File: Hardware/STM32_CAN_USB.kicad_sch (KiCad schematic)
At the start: 28 parts, among them J1 USB_C_Receptacle_USB2.0_14P, J2 SWD, J3 CAN Connector, J4 JP1, SW1 RESET, U1 AP2112K-3.3, U2 STM32F103C8Tx, U3 SN65HVD230, Y1 8Mhz

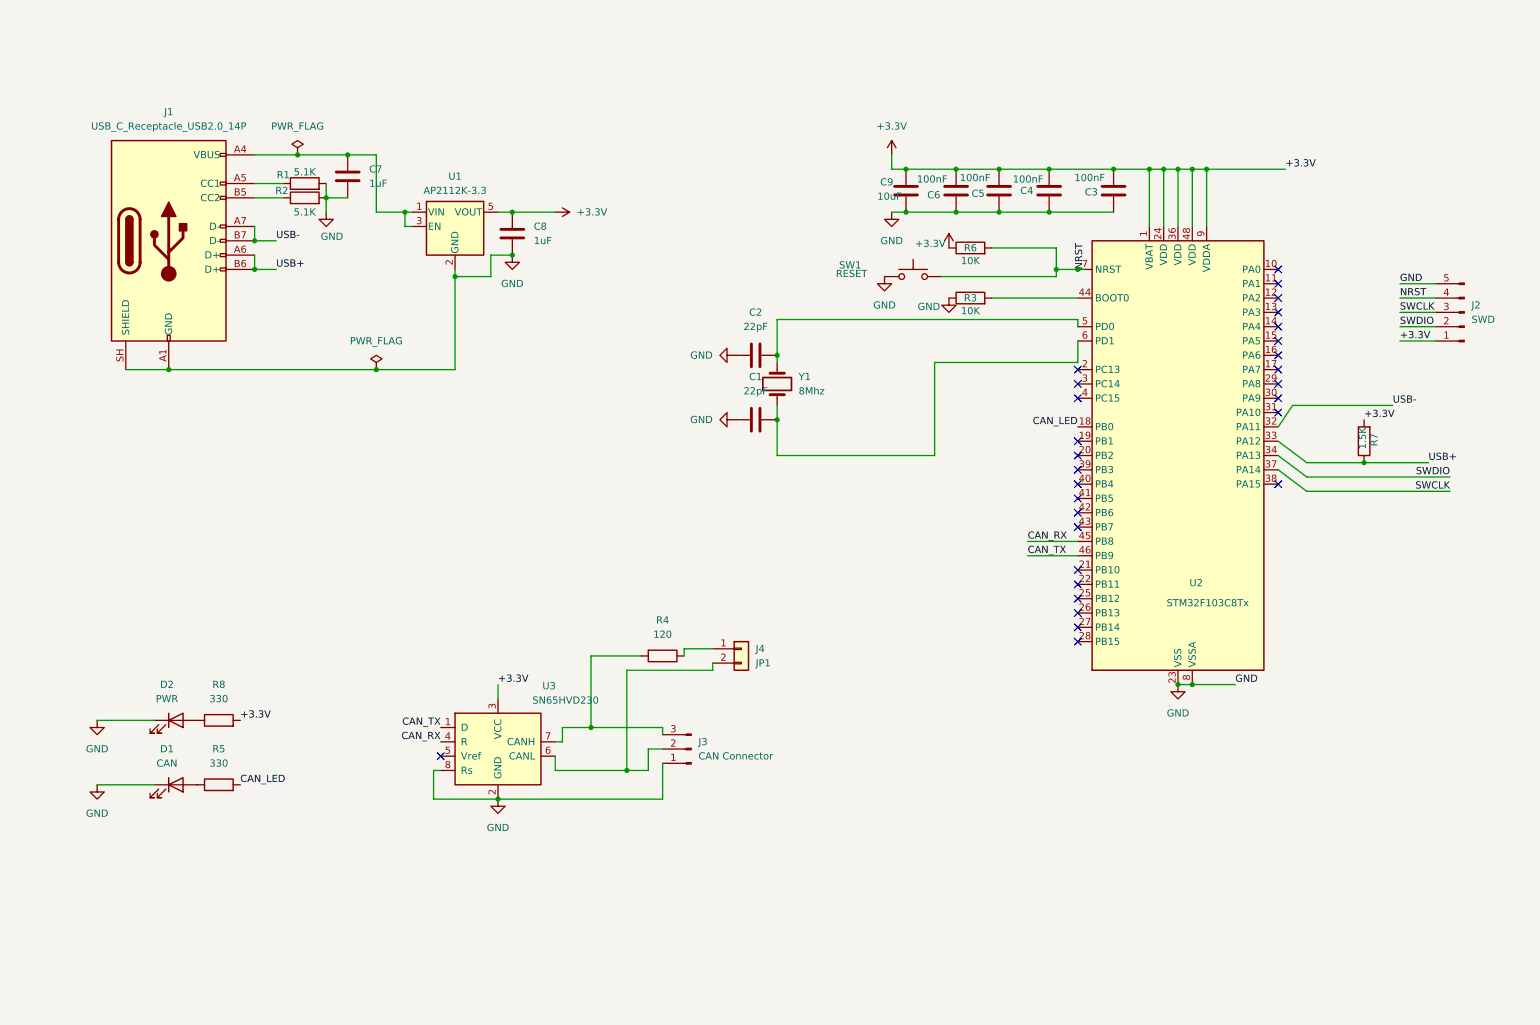
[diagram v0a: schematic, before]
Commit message: Replace project with updated design
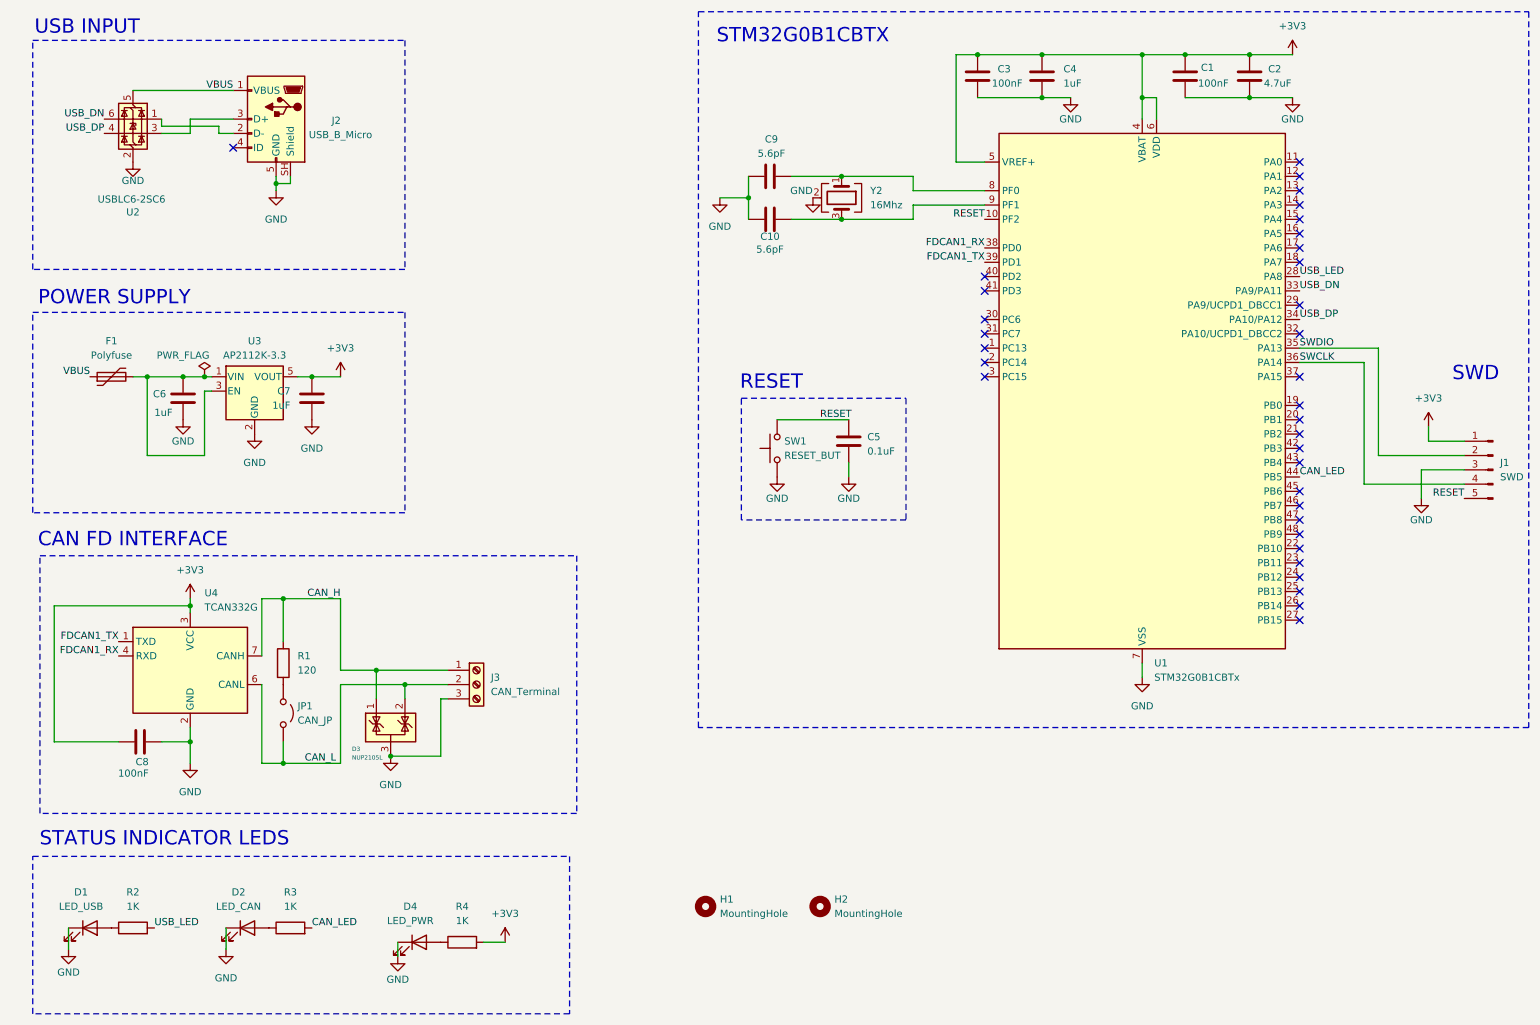
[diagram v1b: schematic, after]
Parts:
- removed J1: USB_C_Receptacle_USB2.0_14P, Connector_USB:USB_C_Receptacle_HRO_TYPE-C-31-M-12, symbol Connector:USB_C_Receptacle_USB2.0_14P
- removed J2: SWD, Connector_PinHeader_2.54mm:PinHeader_1x05_P2.54mm_Vertical, symbol Connector:Conn_01x05_Pin
- removed J3: CAN Connector, TerminalBlock_Phoenix:TerminalBlock_Phoenix_MKDS-1,5-3_1x03_P5.00mm_Horizontal, symbol Connector:Conn_01x03_Pin
- removed J4: JP1, Connector_PinHeader_2.54mm:PinHeader_1x02_P2.54mm_Vertical, symbol Connector_Generic:Conn_01x02
- removed R5, R8: 330, Resistor_SMD:R_0805_2012Metric, symbol Device:R
- removed R6: 10K, Resistor_SMD:R_0805_2012Metric, symbol Device:R
- removed R7: 1.5K, Resistor_SMD:R_0805_2012Metric, symbol Device:R
- removed U1: AP2112K-3.3, Package_TO_SOT_SMD:SOT-23-5, symbol Regulator_Linear:AP2112K-3.3
- removed U2: STM32F103C8Tx, Package_QFP:LQFP-48_7x7mm_P0.5mm, symbol MCU_ST_STM32F1:STM32F103C8Tx
- removed U3: SN65HVD230, Package_SO:SOIC-8_3.9x4.9mm_P1.27mm, symbol Interface_CAN_LIN:SN65HVD230
- removed Y1: 8Mhz, Crystal:Crystal_SMD_3225-4Pin_3.2x2.5mm, symbol Device:Crystal
- added C10: 5.6pF, Capacitor_SMD:C_0603_1608Metric, symbol Device:C
- added D3: NUP2105L, Package_TO_SOT_SMD:SOT-23, symbol Power_Protection:NUP2105L
- added D4: LED_PWR, LED_SMD:LED_0603_1608Metric, symbol Device:LED
- added F1: Polyfuse, Fuse:Fuse_1206_3216Metric, symbol Device:Polyfuse
- added H1, H2: MountingHole, MountingHole:MountingHole_2mm, symbol Mechanical:MountingHole
- added J1: SWD, Connector_PinHeader_2.54mm:PinHeader_1x05_P2.54mm_Vertical, symbol Connector:Conn_01x05_Pin
- added J2: USB_B_Micro, Connector_USB:USB_Micro-B_Amphenol_10118194_Horizontal, symbol Connector:USB_B_Micro
- added J3: CAN_Terminal, TerminalBlock_Phoenix:TerminalBlock_Phoenix_MKDS-1,5-3-5.08_1x03_P5.08mm_Horizontal, symbol Connector:Screw_Terminal_01x03
- added JP1: CAN_JP, Connector_PinHeader_2.54mm:PinHeader_1x02_P2.54mm_Vertical, symbol Jumper:Jumper_2_Open
- added U1: STM32G0B1CBTx, Package_QFP:LQFP-48_7x7mm_P0.5mm, symbol MCU_ST_STM32G0:STM32G0B1CBTx
- added U2: USBLC6-2SC6, Package_TO_SOT_SMD:SOT-23-6, symbol Power_Protection:USBLC6-2SC6
- added U3: AP2112K-3.3, Package_TO_SOT_SMD:SOT-23-5, symbol Regulator_Linear:AP2112K-3.3
- added U4: TCAN332G, Package_SO:SOIC-8_3.9x4.9mm_P1.27mm, symbol Interface_CAN_LIN:TCAN332G
- added Y2: 16Mhz, Crystal:Crystal_SMD_3225-4Pin_3.2x2.5mm, symbol Device:Crystal_GND24
- C1: value 22pF -> 100nF
- C2: value 22pF -> 4.7uF; footprint Capacitor_SMD:C_0603_1608Metric -> Capacitor_SMD:C_0805_2012Metric
- C4, C6: value 100nF -> 1uF
- C5: value 100nF -> 0.1uF
- C8: value 1uF -> 100nF
- C9: value 10uF -> 5.6pF; footprint Capacitor_SMD:C_0805_2012Metric -> Capacitor_SMD:C_0603_1608Metric
- D1: value CAN -> LED_USB; footprint LED_SMD:LED_0805_2012Metric -> LED_SMD:LED_0603_1608Metric
- D2: value PWR -> LED_CAN; footprint LED_SMD:LED_0805_2012Metric -> LED_SMD:LED_0603_1608Metric
- R1: value 5.1K -> 120; footprint Resistor_SMD:R_0805_2012Metric -> Resistor_SMD:R_0603_1608Metric
- R2: value 5.1K -> 1K; footprint Resistor_SMD:R_0805_2012Metric -> Resistor_SMD:R_0603_1608Metric
- R3: value 10K -> 1K; footprint Resistor_SMD:R_0805_2012Metric -> Resistor_SMD:R_0603_1608Metric
- R4: value 120 -> 1K; footprint Resistor_SMD:R_0805_2012Metric -> Resistor_SMD:R_0603_1608Metric
- SW1: value RESET -> RESET_BUT; footprint Button_Switch_SMD:SW_SPST_TL3342 -> Button_Switch_SMD:SW_Push_1P1T_NO_CK_KMR2
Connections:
- net CAN_LED: now also R3.2, U1.44 (PB5)
- net GND: now also C1.2, C3.2, C4.2, C5.2, C6.2, C7.2, C8.2, C10.2, D3.3 (A), D4.1 (K), J1.3 (Pin_3), J2.5 (GND), J2.SH (Shield), J3.3 (Pin_3), U1.7 (VSS), U2.2 (GND), U3.2 (GND), U4.2 (GND), Y2.2 (G), Y2.4 (G); no longer C1.1, C3.1, C4.1, C5.1, C6.1, C7.1, C8.1, R1.2, R2.2, R3.1
- net SWCLK: now also J1.4 (Pin_4), U1.36 (PA14)
- net SWDIO: now also J1.2 (Pin_2), U1.35 (PA13)
- net at R4.1: now also D4.2 (A)
- net +3V3: now reaches R4.2
- net +3V3: now also C1.1, C2.1, C3.1, C4.1, C7.1, C8.1, J1.1 (Pin_1), U1.4 (VBAT), U1.5 (VREF+), U1.6 (VDD), U3.5 (VOUT), U4.3 (VCC)
- net at D1.2 (A): now also R2.1
- net CAN_H: now reaches R1.1
- net CAN_H: now also D3.1 (K), J3.1 (Pin_1), U4.7 (CANH)
- net at D2.2 (A): now also R3.1
- removed net +3.3V: C3.2, C4.2, C5.2, C6.2, C8.2, C9.1
- net NRST renamed RESET
- net RESET: now also C5.1, J1.5 (Pin_5), U1.10 (PF2)
- new net: C9.1, U1.8 (PF0), Y2.1
- new net: C10.1, U1.9 (PF1), Y2.3
- new net: C6.1, F1.2, U3.1 (VIN), U3.3 (EN)
- new net: JP1.1 (A), R1.2
- new net: J2.2 (D-), U2.1 (I/O1)
- new net: J2.3 (D+), U2.3 (I/O2)
- new net CAN_L: D3.2 (K), J3.2 (Pin_2), JP1.2 (B), U4.6 (CANL)
- new net FDCAN1_RX: U1.38 (PD0), U4.4 (RXD)
- new net FDCAN1_TX: U1.39 (PD1), U4.1 (TXD)
- new net USB_DN: U1.33 (PA9/PA11), U2.6 (I/O1)
- new net USB_DP: U1.34 (PA10/PA12), U2.4 (I/O2)
- new net USB_LED: R2.2, U1.28 (PA8)
- new net VBUS: F1.1, J2.1 (VBUS), U2.5 (VBUS)
- no-connect marks 29 -> 34
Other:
- note added: "CAN FD INTERFACE"
- note added: "POWER SUPPLY"
- note added: "RESET"
- note added: "STATUS INDICATOR LEDS"
- note added: "STM32G0B1CBTX"
- note added: "SWD"
- note added: "USB INPUT"
